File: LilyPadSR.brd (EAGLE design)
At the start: 50.9 x 50.9 mm, 40 parts, among them IC1 74HC595D, IC2 74HC595D

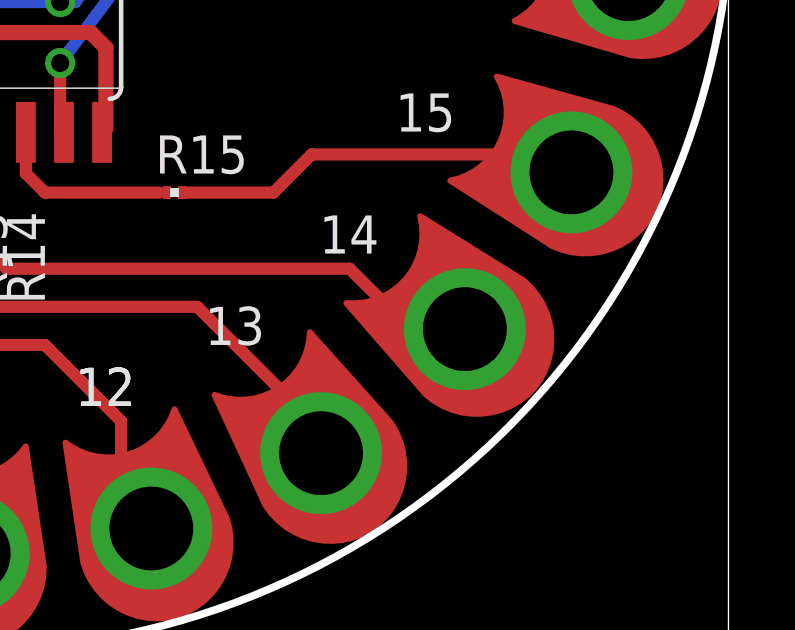
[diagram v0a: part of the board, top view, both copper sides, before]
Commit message: minor fix
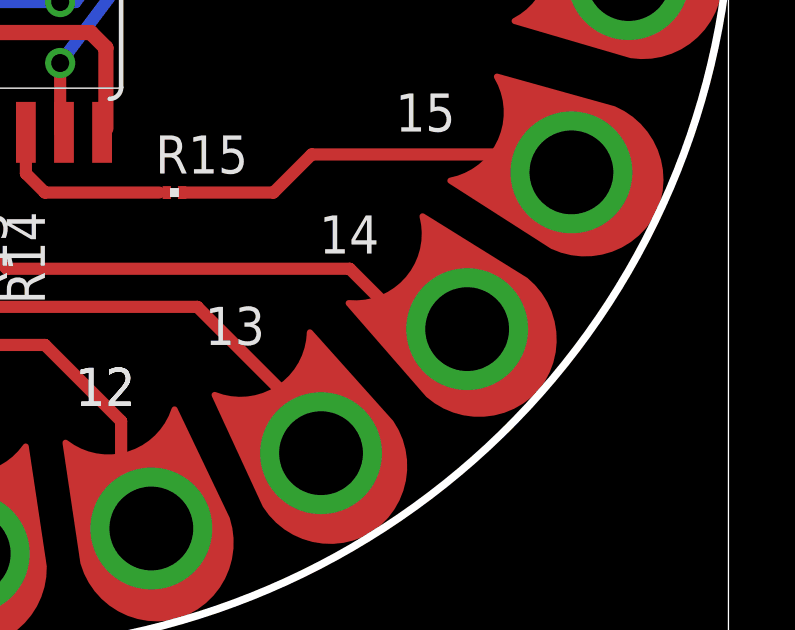
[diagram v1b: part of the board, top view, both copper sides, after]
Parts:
- moved U$15 0.08 mm to (42.0, 39.9)
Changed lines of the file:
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@@
 <element name="U$13" library="LilyPad-Wearables" package="PETAL-LONG-1" value="SEWTAP1" x="31.496" y="33.2232" locked="yes" rot="R107"/>
 <element name="U$14" library="LilyPad-Wearables" package="PETAL-LONG-1" value="SEWTAP1" x="37.1602" y="35.7378" locked="yes" rot="R123.3"/>
-<element name="U$15" library="LilyPad-Wearables" package="PETAL-LONG-1" value="SEWTAP1" x="41.9608" y="39.878" locked="yes" rot="R139.6"/>
+<element name="U$15" library="LilyPad-Wearables" package="PETAL-LONG-1" value="SEWTAP1" x="42.037" y="39.878" locked="yes" rot="R139.6"/>
 <element name="U$16" library="LilyPad-Wearables" package="PETAL-LONG-1" value="SEWTAP1" x="45.5168" y="45.1104" locked="yes" rot="R155.9"/>
 <element name="U$17" library="LilyPad-Wearables" package="PETAL-LONG-1" value="SEWTAP1" x="47.4218" y="51.562" locked="yes" rot="R172.2"/>
@@
 <wire x1="38.1" y1="41.91" x2="39.37" y2="40.64" width="0.4064" layer="1"/>
 <wire x1="39.37" y1="40.64" x2="41.19539375" y2="40.64" width="0.4064" layer="1"/>
-<wire x1="41.19539375" y1="40.64" x2="41.937953125" y2="39.897440625" width="0.4064" layer="1"/>
+<wire x1="41.19539375" y1="40.64" x2="42.014153125" y2="39.897440625" width="0.4064" layer="1"/>
 </signal>
 <signal name="Q15">
